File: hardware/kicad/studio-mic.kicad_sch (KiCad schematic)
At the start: 2 parts, among them Q1 LSK170

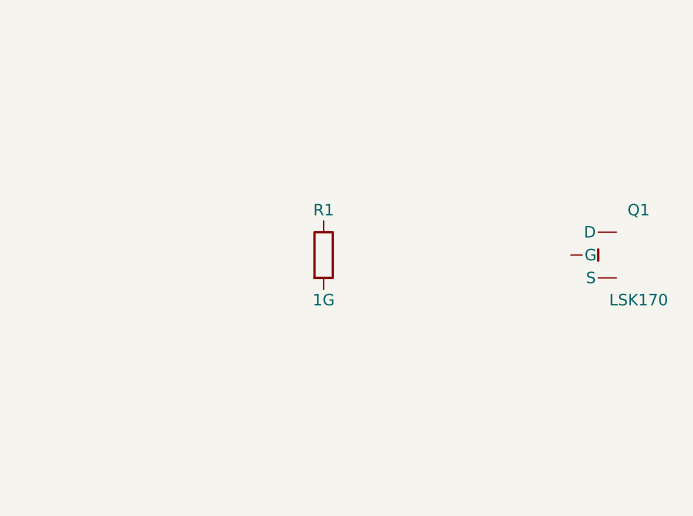
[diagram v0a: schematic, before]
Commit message: (acm) Currently Listening To:  -
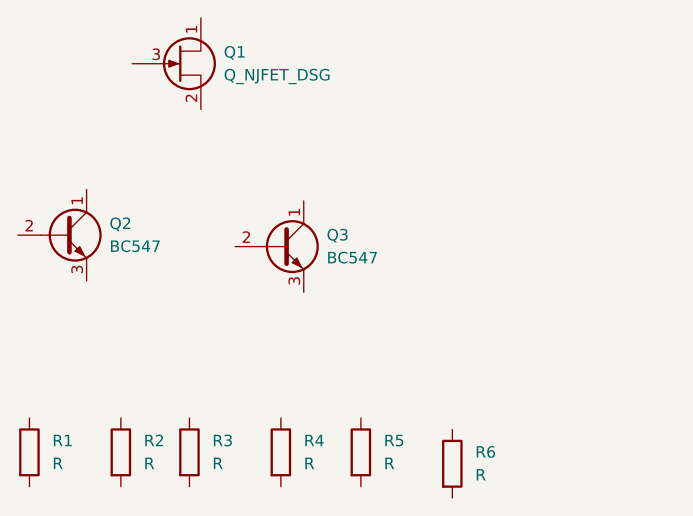
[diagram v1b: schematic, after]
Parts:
- added Q2, Q3: BC547, Package_TO_SOT_THT:TO-92_Inline, symbol Transistor_BJT:BC547
- added R2, R3, R4, R5, R6: R, symbol Device:R
- Q1: value LSK170 -> Q_NJFET_DSG
- R1: value 1G -> R

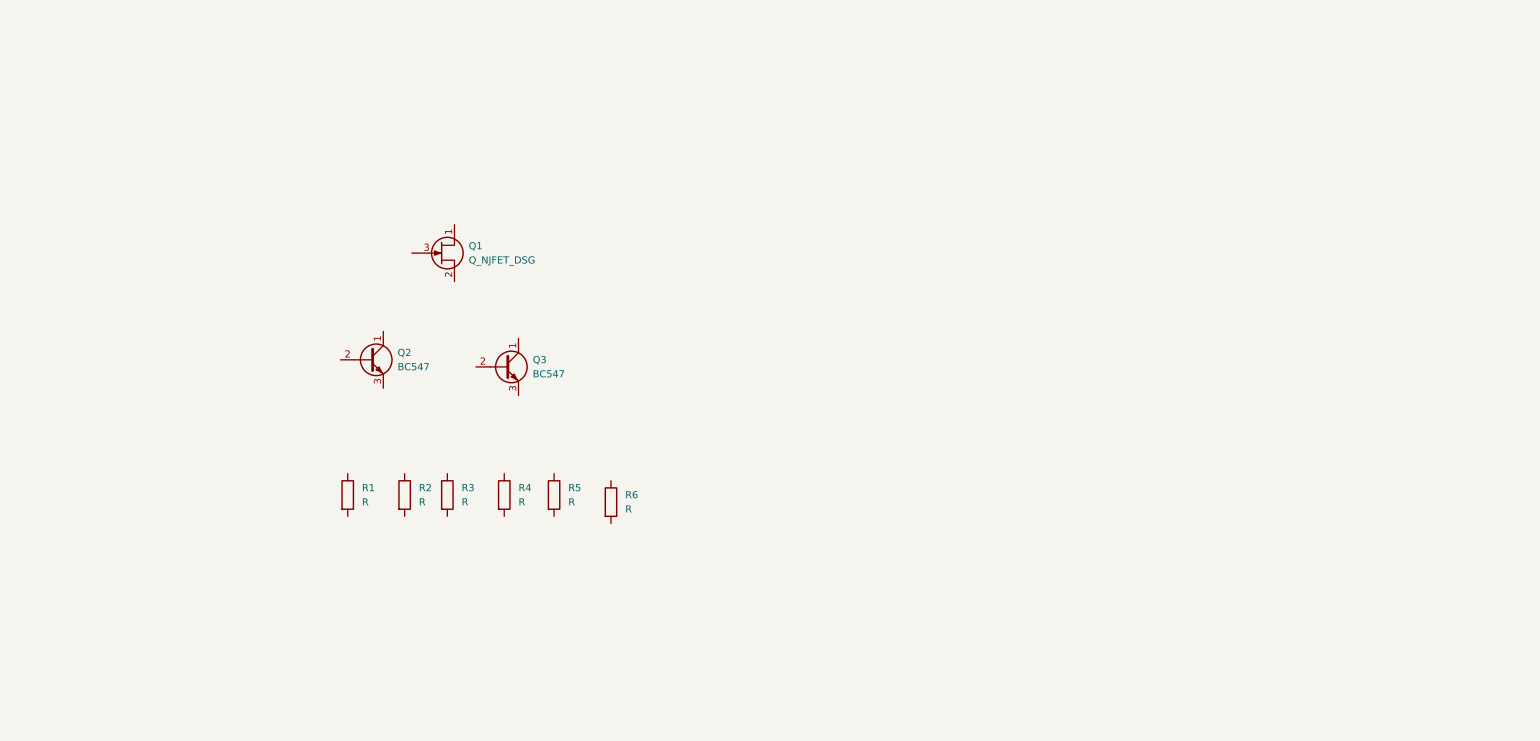
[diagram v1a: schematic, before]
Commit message: (acm) Currently Listening To:  -
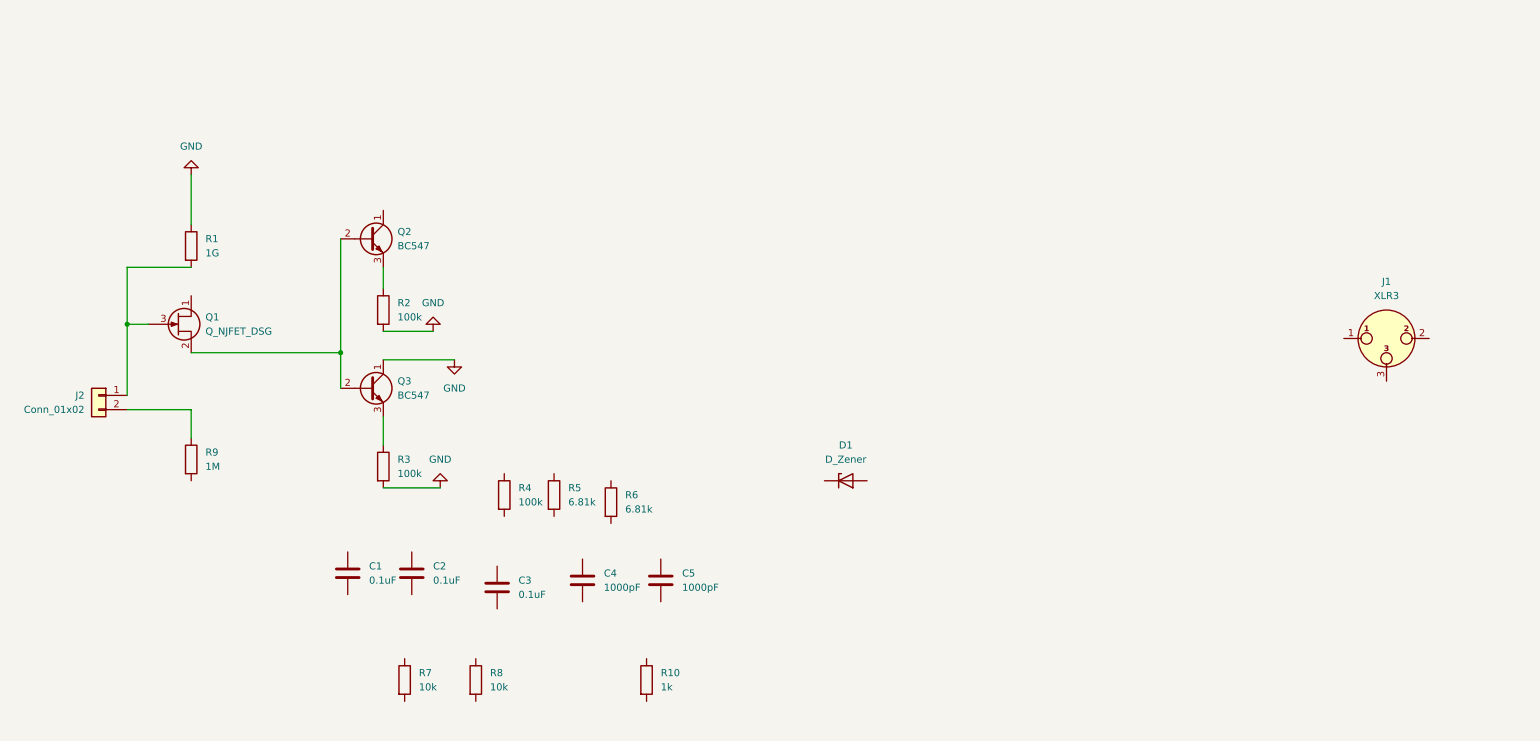
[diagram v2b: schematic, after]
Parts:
- added C1, C2, C3: 0.1uF, symbol Device:C
- added C4, C5: 1000pF, symbol Device:C
- added D1: D_Zener, symbol Device:D_Zener
- added J1: XLR3, symbol Connector_Audio:XLR3
- added J2: Conn_01x02, symbol Connector_Generic:Conn_01x02
- added R10: 1k, symbol Device:R
- added R7, R8: 10k, symbol Device:R
- added R9: 1M, symbol Device:R
- R1: value R -> 1G
- R2, R3, R4: value R -> 100k
- R5, R6: value R -> 6.81k
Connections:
- net at Q2.2 (B): now also Q1.2 (S), Q3.2 (B)
- net at Q2.3 (E): now also R2.1
- net at R3.1: now also Q3.3 (E)
- net GND: now reaches R3.2
- net GND: now also Q3.1 (C), R1.1, R2.2
- net at Q1.3 (G): now also R1.2, J2.1 (Pin_1)
- new net: J2.2 (Pin_2), R9.1
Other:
- moved on the sheet: Q1, Q2, Q3, R1, R2, R3

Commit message: (acm) Currently Listening To:  -
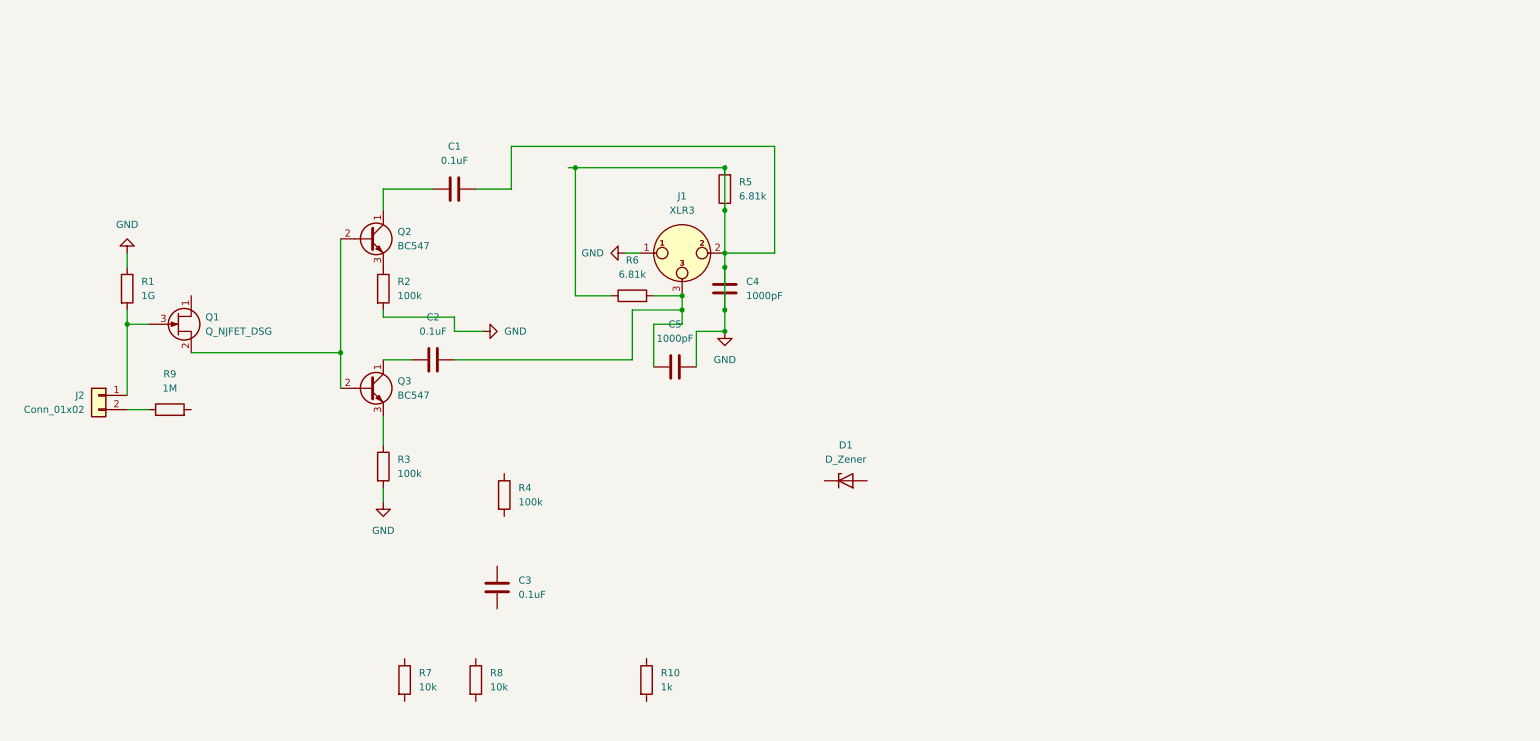
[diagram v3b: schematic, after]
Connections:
- net GND: now also C1.2, C4.1, C4.2, C5.2, J1.1, J1.2, R5.1, R5.2, R6.1; no longer Q3.1 (C)
- net at C1.1: now also Q2.1 (C)
- net at R6.2: now also C2.2, C5.1, J1.3
- net at C2.1: now also Q3.1 (C)
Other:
- moved on the sheet: C1, C2, C4, C5, J1, R1, R2, R5, R6, R9

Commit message: (acm) Currently Listening To:  -
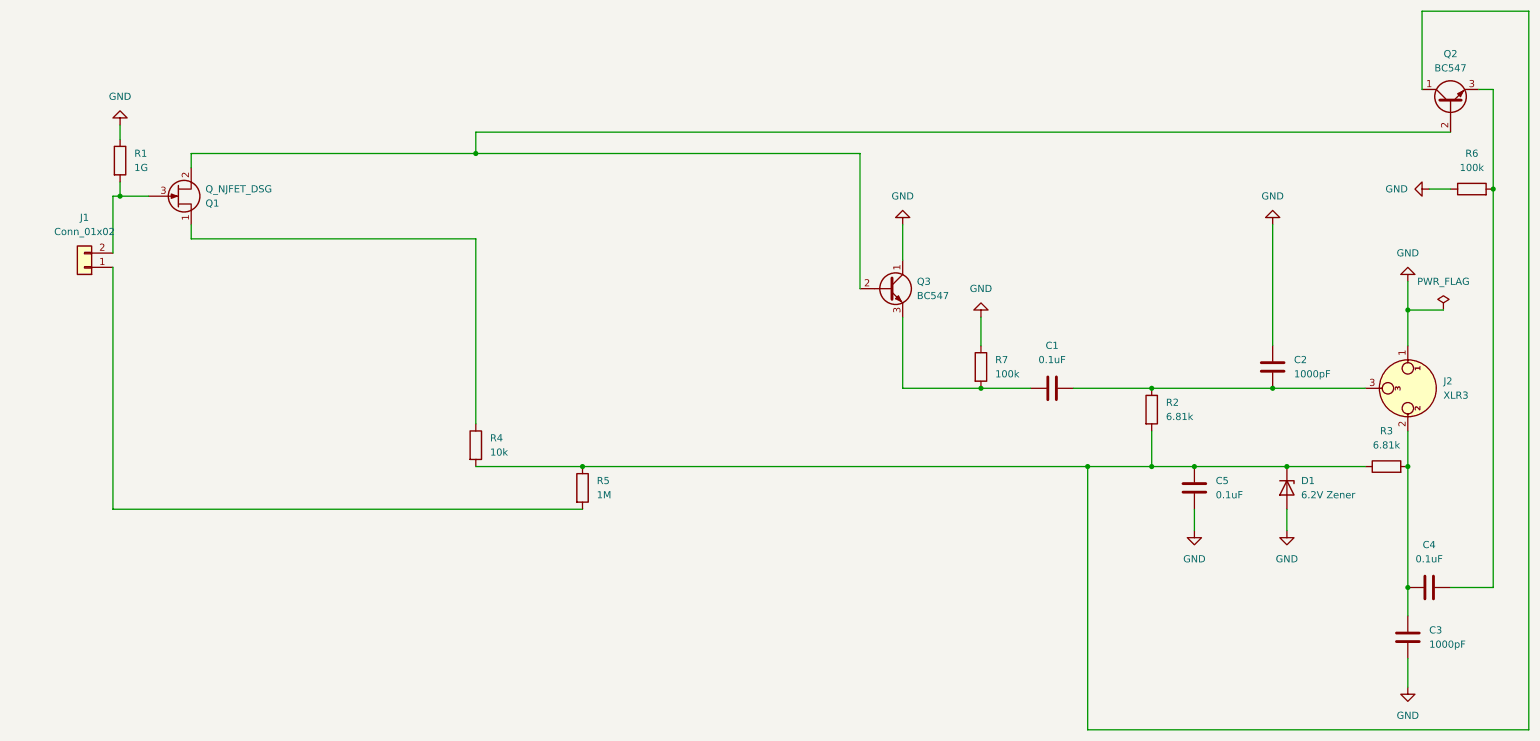
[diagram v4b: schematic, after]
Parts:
- removed J1: XLR3, symbol Connector_Audio:XLR3
- removed J2: Conn_01x02, symbol Connector_Generic:Conn_01x02
- removed R10: 1k, symbol Device:R
- removed R8: 10k, symbol Device:R
- removed R9: 1M, symbol Device:R
- added J1: Conn_01x02, symbol Connector_Generic:Conn_01x02
- added J2: XLR3, symbol Connector_Audio:XLR3
- C2, C3: value 0.1uF -> 1000pF
- C4, C5: value 1000pF -> 0.1uF
- D1: value D_Zener -> 6.2V Zener
- R2, R3: value 100k -> 6.81k
- R4: value 100k -> 10k
- R5: value 6.81k -> 1M
- R6: value 6.81k -> 100k
- R7: value 10k -> 100k
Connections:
- net GND: now also C2.1, C3.2, D1.2 (A), Q3.1 (C), R7.1, J2.1; no longer C1.2, C4.1, C4.2, R2.2, R3.2, R5.1, R5.2
- net at Q2.1 (C): now also C5.1, D1.1 (K), R2.2, R3.1, R4.2, R5.1; no longer C1.1
- net at Q2.3 (E): now also C4.2, R6.2; no longer R2.1
- net at Q3.3 (E): now also C1.1, R7.2; no longer R3.1
- net at C3.1: now also C4.1, R3.2, J2.2
- net at Q1.1 (D): now also R4.1
- net at Q1.3 (G), R1.2: now also J1.2 (Pin_2)
- new net: C1.2, C2.2, J2.3, R2.1
- new net: J1.1 (Pin_1), R5.2
